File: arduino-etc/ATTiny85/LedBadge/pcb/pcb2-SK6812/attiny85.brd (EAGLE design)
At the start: 34 x 34 mm, 19 parts, among them SW1 bat+, SW2 POWER

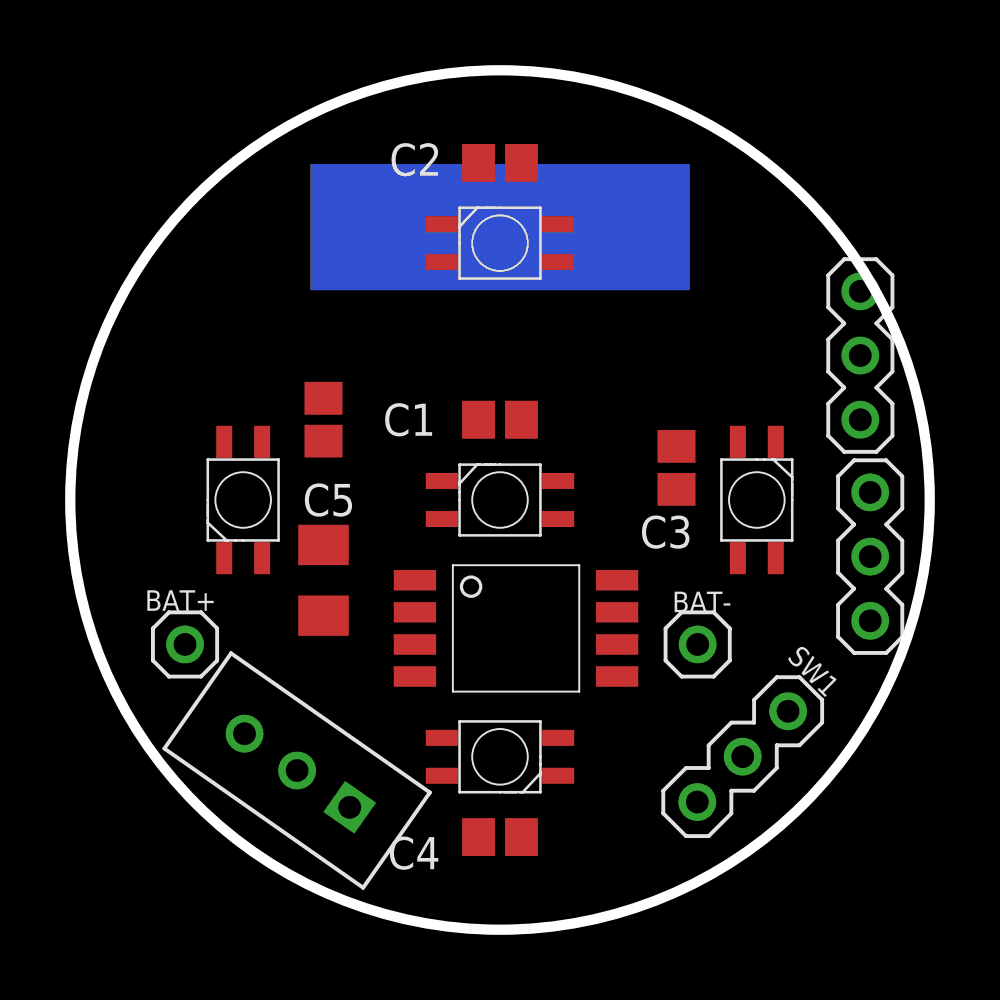
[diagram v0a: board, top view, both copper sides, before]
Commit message: UPD: pcb2-SK6812/
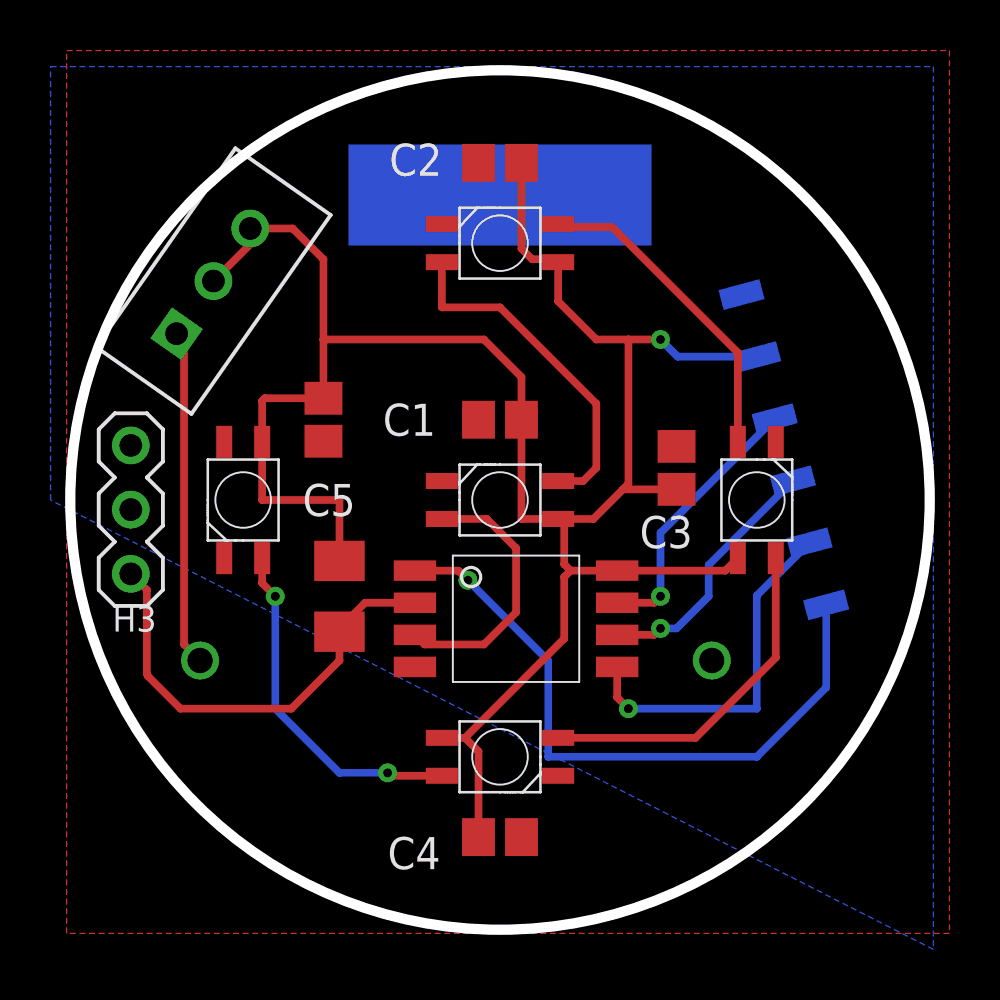
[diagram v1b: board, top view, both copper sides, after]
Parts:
- removed BAT+: bat+, ytani1:PINHEAD-MA01-1
- removed BAT-: bat-, ytani1:PINHEAD-MA01-1
- removed SV1: PIN-A, ytani1:PINHEAD-MA03-1
- removed SV2: PIN-B, ytani1:PINHEAD-MA03-1
- removed SW1: bat+, ytani1:PINHEAD-MA03-1
- added BAT1: (no value), ytani1:BAT-CR2032-1
- added H1, H2: (no value), ytani1:PINHEAD-MA03-2
- added H3: (no value), ytani1:PINHEAD-MA03-1
- PAD33: value PAD150X50 -> PAD12X4; device ytani1:PAD5X15 -> ytani1:PAD-12X4
- moved SW2 19.7 mm to (6.99, 27.9), turned to 55 degrees
- moved PAD33 1.27 mm to (19.1, 32.4)
- moved R1 0.90 mm to (12.7, 16.5)
- moved ATTINY85-1 0.38 mm to (19.7, 15.6)
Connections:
- net +3V3: now also BAT1.BAT+; no longer BAT+.1
- net BAT+: now also H2.2; no longer SV2.2
- net GND: now also BAT1.BAT-, H2.3, H3.1; no longer BAT-.1, SV2.3, SW1.1, SW1.2
- net N$2: now also H2.1; no longer SV2.1
- net N$3: now also H1.3; no longer SV1.3
- net N$4: now also H1.1; no longer SV1.1
- net N$5: now also H1.2; no longer SV1.2
- net PB3: now also H3.3; no longer SW1.3
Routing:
- net BAT+: track 0.61 -> 88.0 mm, vias 0 -> 1
- net N$4: track 0.00 -> 26.0 mm, vias 0 -> 1
- net PB3: track 0.13 -> 17.9 mm
- net N$5: track 0.00 -> 14.3 mm, vias 0 -> 1
- net N$9: track 0.00 -> 13.9 mm, vias 0 -> 2
- net N$6: track 0.00 -> 13.7 mm
- net N$8: track 0.12 -> 13.9 mm
- net +3V3: track 0.00 -> 13.3 mm
- net N$7: track 0.00 -> 12.7 mm
- net N$2: track 0.00 -> 10.7 mm, vias 0 -> 1
- net N$1: track 0.00 -> 10.6 mm
- net N$3: track 0.00 -> 10.2 mm, vias 0 -> 1
- added copper zone on layer 1, net GND
- added copper zone on layer 16, net GND
